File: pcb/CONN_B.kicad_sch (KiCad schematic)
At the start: 8 parts, among them J2 USB_B, J3 6437288-4, J4 Conn_ARM_SWD_TagConnect_TC2030

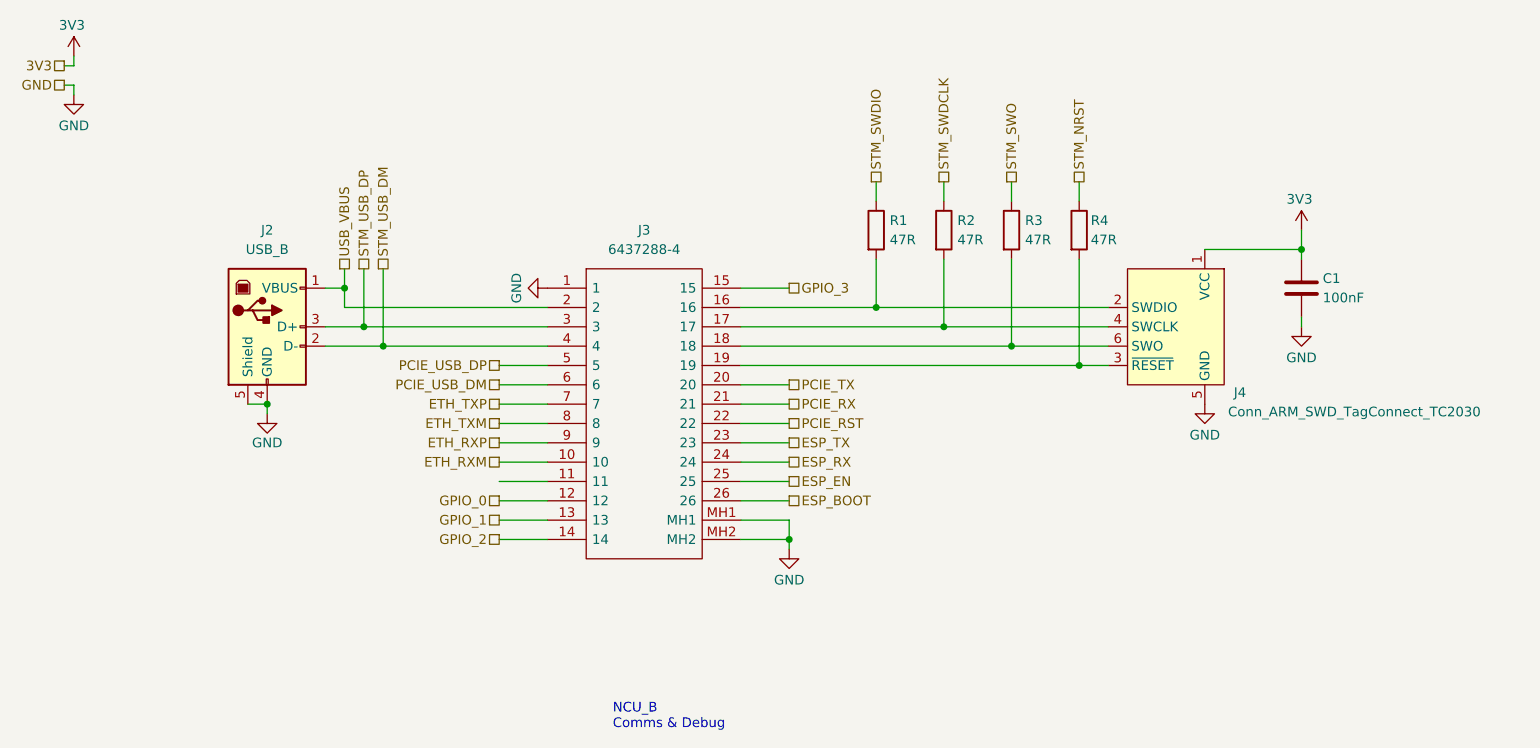
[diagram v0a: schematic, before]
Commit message: power done
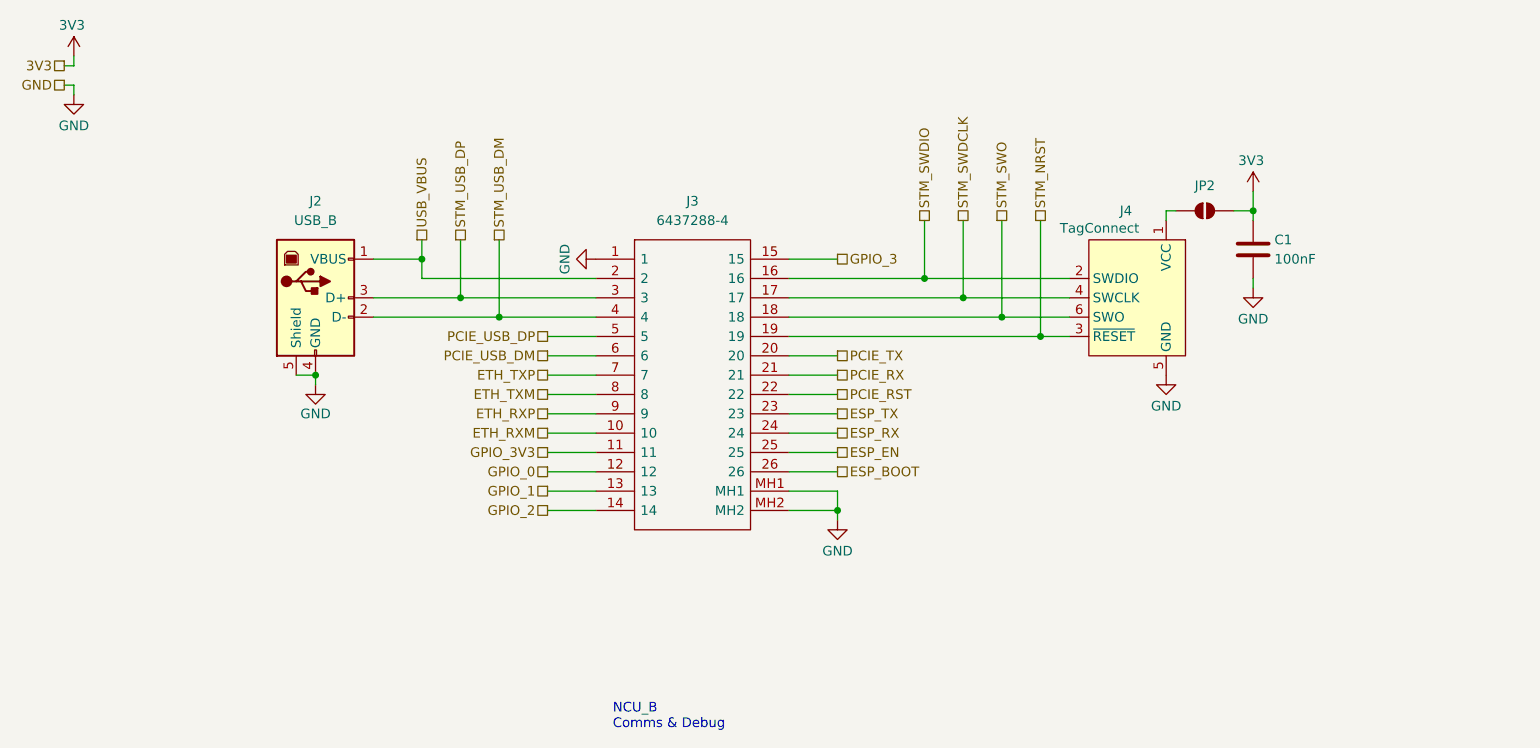
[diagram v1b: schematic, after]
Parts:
- removed R1, R2, R3, R4: 47R, Resistor_SMD:R_0603_1608Metric_Pad0.98x0.95mm_HandSolder, symbol Device:R
- added JP2: SolderJumper_2_Open, symbol Jumper:SolderJumper_2_Open
- J4: value Conn_ARM_SWD_TagConnect_TC2030 -> TagConnect
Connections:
- net 3V3: now also JP2.2 (B); no longer J4.1 (VCC)
- net STM_NRST: now also J3.19, J4.3 (~{RESET})
- net STM_SWDCLK: now also J3.17, J4.4 (SWCLK)
- net STM_SWDIO: now also J3.16, J4.2 (SWDIO)
- net STM_SWO: now also J3.18, J4.6 (SWO)
- net GPIO_3V3: now reaches J3.11
- new net: J4.1 (VCC), JP2.1 (A)
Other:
- moved on the sheet: C1, J2, J3, J4
